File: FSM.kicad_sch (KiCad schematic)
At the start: 10 parts, among them SW2 SW_Push, U10 40106, U22 74HCT00, U23 74HCT74, U24 74HCT00, U9 74HCT04

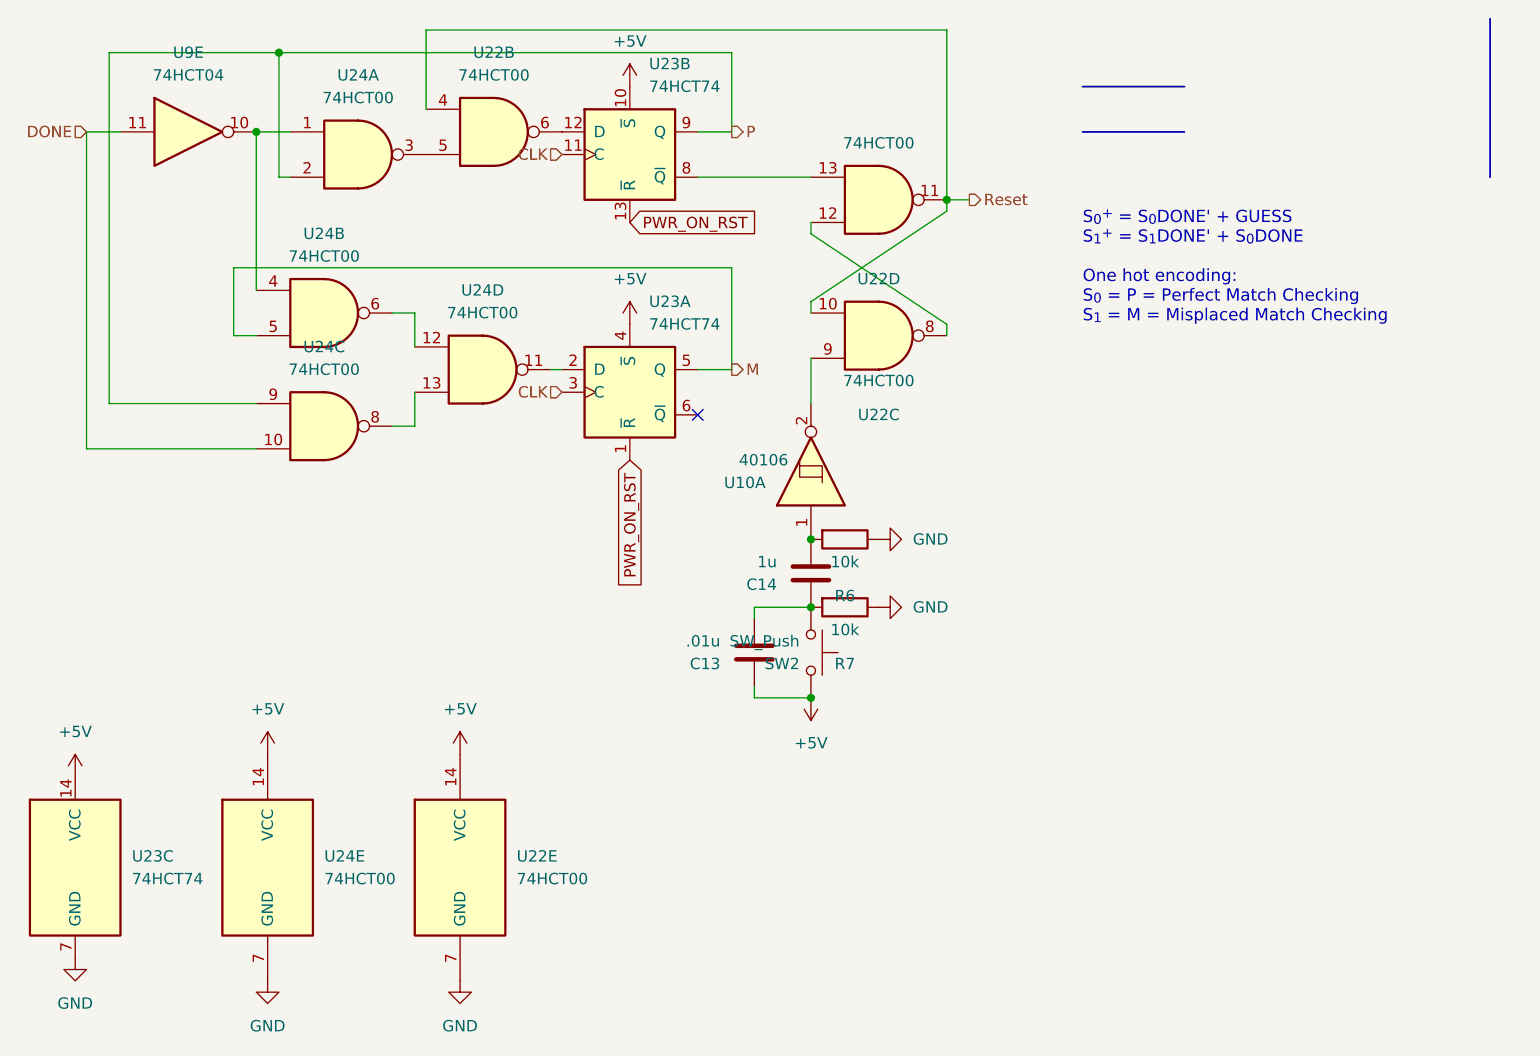
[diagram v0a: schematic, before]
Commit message: routed
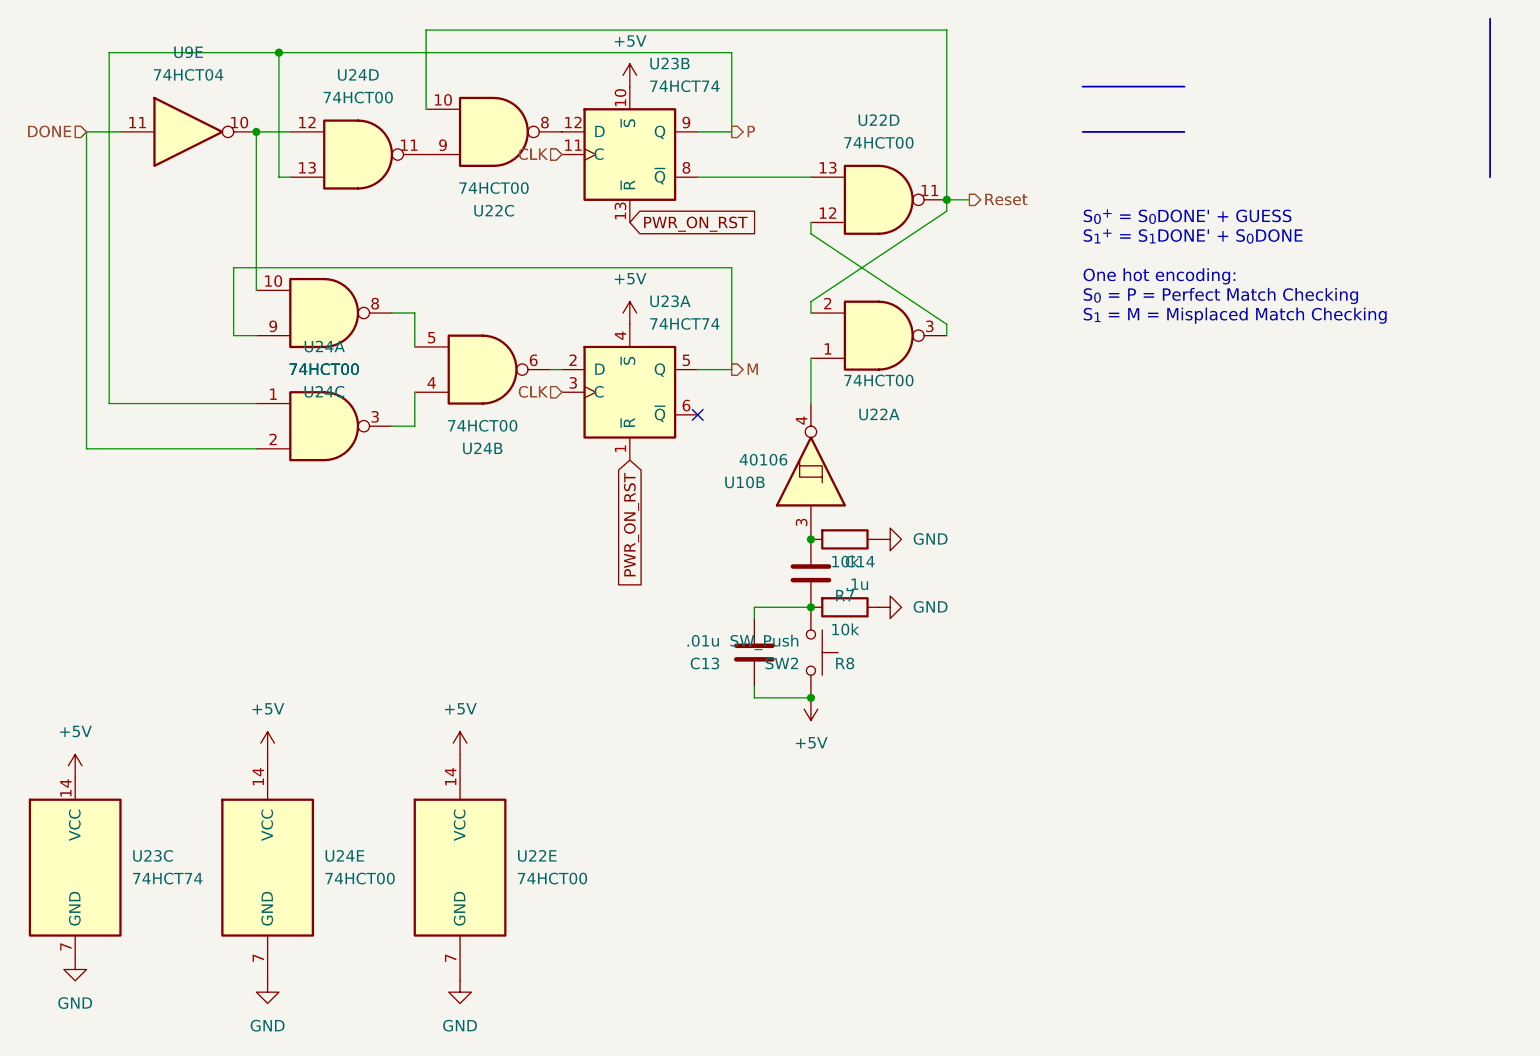
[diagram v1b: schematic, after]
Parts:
- C14: value 1u -> .1u
- renumbered R6 to R7, R7 to R8
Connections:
- net DONE: now also U24.2; no longer U24.10
- net M: now also U24.9; no longer U24.5
- net P: now also U24.1, U24.13; no longer U24.2, U24.9
- net Reset: now also U22.10, U22.2; no longer U22.10, U22.4
- net at C14.2, R7.2: now also U10.3; no longer U10.1
- net at U22.12: now also U22.3; no longer U22.8
- net at U23.12 (D): now also U22.8; no longer U22.6
- net at U23.2 (D): now also U24.6; no longer U24.11
- new net: U10.4, U22.1
- new net: U24.3, U24.4
- new net: U22.9, U24.11
- new net: U24.10, U24.12, U9.10
- new net: U24.5, U24.8
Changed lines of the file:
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@@
 		(on_board yes)
 		(dnp no)
-		(property "Reference" "R6"
+		(property "Reference" "R7"
 			(at 106.68 82.55 90)
 			(effects
@@
 			(project "ECE145Mastermind"
 				(path "/8c64fe8a-5d6b-41bc-b3a3-9bda7b2e0f2c/c249946c-91e3-42cd-8f8a-d6059405d3e8"
-					(reference "R6")
+					(reference "R7")
 					(unit 1)
 				)
@@
 		(at 110.49 53.34 0)
 		(mirror x)
-		(unit 3)
+		(unit 1)
 		(exclude_from_sim no)
 		(in_bom yes)
@@
 				(path "/8c64fe8a-5d6b-41bc-b3a3-9bda7b2e0f2c/c249946c-91e3-42cd-8f8a-d6059405d3e8"
 					(reference "U22")
-					(unit 3)
+					(unit 1)
 				)
 			)
@@
 		(lib_id "74xx:74HCT00")
 		(at 48.26 63.5 0)
-		(unit 3)
+		(unit 1)
 		(exclude_from_sim no)
 		(in_bom yes)
@@
 				(path "/8c64fe8a-5d6b-41bc-b3a3-9bda7b2e0f2c/c249946c-91e3-42cd-8f8a-d6059405d3e8"
 					(reference "U24")
-					(unit 3)
+					(unit 1)
 				)
 			)
@@
 		(dnp no)
 		(fields_autoplaced yes)
-		(property "Reference" "#PWR075"
+		(property "Reference" "#PWR076"
 			(at 20.32 95.25 0)
 			(effects
@@
 			(project ""
 				(path "/8c64fe8a-5d6b-41bc-b3a3-9bda7b2e0f2c/c249946c-91e3-42cd-8f8a-d6059405d3e8"
-					(reference "#PWR075")
+					(reference "#PWR076")
 					(unit 1)
 				)
@@
 		(lib_id "74xx:74HCT00")
 		(at 67.31 30.48 0)
-		(unit 2)
-		(exclude_from_sim no)
-		(in_bom yes)
-		(on_board yes)
-		(dnp no)
-		(fields_autoplaced yes)
+		(mirror x)
+		(unit 3)
+		(exclude_from_sim no)
+		(in_bom yes)
+		(on_board yes)
+		(dnp no)
 		(property "Reference" "U22"
-			(at 67.3017 21.59 0)
+			(at 67.3017 39.37 0)
 			(effects
 				(font
@@
 		)
 		(property "Value" "74HCT00"
-			(at 67.3017 24.13 0)
+			(at 67.3017 36.83 0)
 			(effects
 				(font
@@
 				(path "/8c64fe8a-5d6b-41bc-b3a3-9bda7b2e0f2c/c249946c-91e3-42cd-8f8a-d6059405d3e8"
 					(reference "U22")
-					(unit 2)
+					(unit 3)
 				)
 			)
@@
 		(dnp no)
 		(fields_autoplaced yes)
-		(property "Reference" "#PWR080"
+		(property "Reference" "#PWR081"
 			(at 63.5 132.08 0)
 			(effects
@@
 			(project "ECE145Mastermind"
 				(path "/8c64fe8a-5d6b-41bc-b3a3-9bda7b2e0f2c/c249946c-91e3-42cd-8f8a-d6059405d3e8"
-					(reference "#PWR080")
+					(reference "#PWR081")
 					(unit 1)
 				)
@@
 		(fields_autoplaced yes)
 		(property "Reference" "C14"
-			(at 99.06 81.2801 0)
-			(effects
-				(font
-					(size 1.27 1.27)
-				)
-				(justify left)
-			)
-		)
-		(property "Value" "1u"
-			(at 99.06 78.7401 0)
-			(effects
-				(font
-					(size 1.27 1.27)
-				)
-				(justify left)
+			(at 106.68 78.7399 0)
+			(effects
+				(font
+					(size 1.27 1.27)
+				)
+				(justify right)
+			)
+		)
+		(property "Value" ".1u"
+			(at 106.68 81.2799 0)
+			(effects
+				(font
+					(size 1.27 1.27)
+				)
+				(justify right)
 			)
 		)
@@
 		(dnp no)
 		(fields_autoplaced yes)
-		(property "Reference" "#PWR084"
+		(property "Reference" "#PWR085"
 			(at 116.84 76.2 0)
 			(effects
@@
 			(project "ECE145Mastermind"
 				(path "/8c64fe8a-5d6b-41bc-b3a3-9bda7b2e0f2c/c249946c-91e3-42cd-8f8a-d6059405d3e8"
-					(reference "#PWR084")
+					(reference "#PWR085")
 					(unit 1)
 				)
@@
 		(dnp no)
 		(fields_autoplaced yes)
-		(property "Reference" "#PWR082"
+		(property "Reference" "#PWR083"
 			(at 82.55 55.88 0)
 			(effects
@@
 			(project ""
 				(path "/8c64fe8a-5d6b-41bc-b3a3-9bda7b2e0f2c/c249946c-91e3-42cd-8f8a-d6059405d3e8"
-					(reference "#PWR082")
+					(reference "#PWR083")
 					(unit 1)
 				)
@@
 		(dnp no)
 		(fields_autoplaced yes)
-		(property "Reference" "#PWR078"
+		(property "Reference" "#PWR079"
 			(at 41.91 132.08 0)
 			(effects
@@
 			(project ""
 				(path "/8c64fe8a-5d6b-41bc-b3a3-9bda7b2e0f2c/c249946c-91e3-42cd-8f8a-d6059405d3e8"
-					(reference "#PWR078")
+					(reference "#PWR079")
 					(unit 1)
 				)
@@
 		(dnp no)
 		(fields_autoplaced yes)
-		(property "Reference" "#PWR076"
+		(property "Reference" "#PWR077"
 			(at 20.32 129.54 0)
 			(effects
@@
 			(project ""
 				(path "/8c64fe8a-5d6b-41bc-b3a3-9bda7b2e0f2c/c249946c-91e3-42cd-8f8a-d6059405d3e8"
-					(reference "#PWR076")
+					(reference "#PWR077")
 					(unit 1)
 				)
@@
 		(fields_autoplaced yes)
 		(property "Reference" "U22"
-			(at 110.4817 46.99 0)
+			(at 110.4817 29.21 0)
 			(effects
 				(font
@@
 		(dnp no)
 		(fields_autoplaced yes)
-		(property "Reference" "#PWR083"
+		(property "Reference" "#PWR084"
 			(at 102.87 101.6 0)
 			(effects
@@
 			(project "ECE145Mastermind"
 				(path "/8c64fe8a-5d6b-41bc-b3a3-9bda7b2e0f2c/c249946c-91e3-42cd-8f8a-d6059405d3e8"
-					(reference "#PWR083")
+					(reference "#PWR084")
 					(unit 1)
 				)
@@
 		(dnp no)
 		(fields_autoplaced yes)
-		(property "Reference" "#PWR079"
+		(property "Reference" "#PWR080"
 			(at 63.5 104.14 0)
 			(effects
@@
 			(project "ECE145Mastermind"
 				(path "/8c64fe8a-5d6b-41bc-b3a3-9bda7b2e0f2c/c249946c-91e3-42cd-8f8a-d6059405d3e8"
-					(reference "#PWR079")
+					(reference "#PWR080")
 					(unit 1)
 				)
@@
 		(dnp no)
 		(fields_autoplaced yes)
-		(property "Reference" "#PWR077"
+		(property "Reference" "#PWR078"
 			(at 41.91 104.14 0)
 			(effects
@@
 			(project ""
 				(path "/8c64fe8a-5d6b-41bc-b3a3-9bda7b2e0f2c/c249946c-91e3-42cd-8f8a-d6059405d3e8"
-					(reference "#PWR077")
+					(reference "#PWR078")
 					(unit 1)
 				)
@@
 		(on_board yes)
 		(dnp no)
-		(property "Reference" "R7"
+		(property "Reference" "R8"
 			(at 106.68 90.17 90)
 			(effects
@@
 			(project "ECE145Mastermind"
 				(path "/8c64fe8a-5d6b-41bc-b3a3-9bda7b2e0f2c/c249946c-91e3-42cd-8f8a-d6059405d3e8"
-					(reference "R7")
+					(reference "R8")
 					(unit 1)
 				)
@@
 		(lib_id "4xxx:40106")
 		(at 102.87 68.58 90)
-		(unit 1)
+		(unit 2)
 		(exclude_from_sim no)
 		(in_bom yes)
@@
 				(path "/8c64fe8a-5d6b-41bc-b3a3-9bda7b2e0f2c/c249946c-91e3-42cd-8f8a-d6059405d3e8"
 					(reference "U10")
-					(unit 1)
+					(unit 2)
 				)
 			)
@@
 		(lib_id "74xx:74HCT00")
 		(at 66.04 57.15 0)
-		(unit 4)
-		(exclude_from_sim no)
-		(in_bom yes)
-		(on_board yes)
-		(dnp no)
-		(fields_autoplaced yes)
+		(mirror x)
+		(unit 2)
+		(exclude_from_sim no)
+		(in_bom yes)
+		(on_board yes)
+		(dnp no)
 		(property "Reference" "U24"
-			(at 66.0317 48.26 0)
+			(at 66.0317 66.04 0)
 			(effects
 				(font
@@
 		)
 		(property "Value" "74HCT00"
-			(at 66.0317 50.8 0)
+			(at 66.0317 63.5 0)
 			(effects
 				(font
@@
 				(path "/8c64fe8a-5d6b-41bc-b3a3-9bda7b2e0f2c/c249946c-91e3-42cd-8f8a-d6059405d3e8"
 					(reference "U24")
-					(unit 4)
+					(unit 2)
 				)
 			)
@@
 		(dnp no)
 		(fields_autoplaced yes)
-		(property "Reference" "#PWR085"
+		(property "Reference" "#PWR086"
 			(at 116.84 83.82 0)
 			(effects
@@
 			(project "ECE145Mastermind"
 				(path "/8c64fe8a-5d6b-41bc-b3a3-9bda7b2e0f2c/c249946c-91e3-42cd-8f8a-d6059405d3e8"
-					(reference "#PWR085")
+					(reference "#PWR086")
 					(unit 1)
 				)
@@
 		(lib_id "74xx:74HCT00")
 		(at 52.07 33.02 0)
-		(unit 1)
+		(unit 4)
 		(exclude_from_sim no)
 		(in_bom yes)
@@
 				(path "/8c64fe8a-5d6b-41bc-b3a3-9bda7b2e0f2c/c249946c-91e3-42cd-8f8a-d6059405d3e8"
 					(reference "U24")
-					(unit 1)
+					(unit 4)
 				)
 			)
@@
 		(lib_id "74xx:74HCT00")
 		(at 48.26 50.8 0)
-		(unit 2)
-		(exclude_from_sim no)
-		(in_bom yes)
-		(on_board yes)
-		(dnp no)
-		(fields_autoplaced yes)
+		(mirror x)
+		(unit 3)
+		(exclude_from_sim no)
+		(in_bom yes)
+		(on_board yes)
+		(dnp no)
 		(property "Reference" "U24"
-			(at 48.2517 41.91 0)
+			(at 48.2517 59.69 0)
 			(effects
 				(font
@@
 		)
 		(property "Value" "74HCT00"
-			(at 48.2517 44.45 0)
+			(at 48.2517 57.15 0)
 			(effects
 				(font
@@
 				(path "/8c64fe8a-5d6b-41bc-b3a3-9bda7b2e0f2c/c249946c-91e3-42cd-8f8a-d6059405d3e8"
 					(reference "U24")
-					(unit 2)
+					(unit 3)
 				)
 			)
@@
 		(dnp no)
 		(fields_autoplaced yes)
-		(property "Reference" "#PWR081"
+		(property "Reference" "#PWR082"
 			(at 82.55 29.21 0)
 			(effects
@@
 			(project ""
 				(path "/8c64fe8a-5d6b-41bc-b3a3-9bda7b2e0f2c/c249946c-91e3-42cd-8f8a-d6059405d3e8"
-					(reference "#PWR081")
+					(reference "#PWR082")
 					(unit 1)
 				)

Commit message: Ground and Power Plane?
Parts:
- SW2: footprint Button_Switch_SMD:SW_SPST_Omron_B3FS-105xP -> Button_Switch_THT:SW_SPST_Omron_B3F-40xx
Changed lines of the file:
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@@
 			)
 		)
-		(property "Footprint" "Button_Switch_SMD:SW_SPST_Omron_B3FS-105xP"
+		(property "Footprint" "Button_Switch_THT:SW_SPST_Omron_B3F-40xx"
 			(at 107.95 88.9 0)
 			(effects
